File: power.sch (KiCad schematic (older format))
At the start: 60 parts, among them J5 VJ1, U1 LFE5U-85F-6BG381C, U3 TLV62569DBV, U4 TLV62569DBV, U5 TLV62569DBV

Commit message: Sync sch and pcb
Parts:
- removed D12: BAT54W, Diode_SMD:D_SOD-323_HandSoldering, symbol Device:D_Schottky
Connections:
- net labels removed: FTDI_nSUSPEND
- wire segments 395 -> 391
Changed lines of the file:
@@
 	7450 4700 6950 4700
 Wire Wire Line
-	3950 4950 4100 4950
-Wire Wire Line
 	4100 1050 4200 1050
 Wire Wire Line
@@
 Wire Wire Line
 	4850 4950 4850 4850
-Wire Wire Line
-	4100 4950 4100 5050
-Connection ~ 4100 4950
-Wire Wire Line
-	2850 4950 3650 4950
 Wire Wire Line
 	7750 1050 7750 1150
@@
 Wire Wire Line
 	2500 4950 2550 4950
-Text Label 2900 4950 0    60   ~ 0
-FTDI_nSUSPEND
 $Comp
 L Device:C C17
@@
 	1    0    0    -1
 $EndComp
-$Comp
-L Device:D_Schottky D12
-U 1 1 5AF673FF
-P 3800 4950
-F 0 "D12" H 3800 5050 50  0000 C CNN
-F 1 "BAT54W" H 3800 4850 50  0000 C CNN
-F 2 "Diode_SMD:D_SOD-323_HandSoldering" H 3800 4950 50  0001 C CNN
-F 3 "" H 3800 4950 50  0001 C CNN
-	1    3800 4950
-	-1   0    0    1
-$EndComp
 Text Notes 850  5050 0    60   ~ 0
 FTDI_nSLEEP is 2.5V\nD12 must be schottky
@@
 Wire Wire Line
 	2900 3700 2900 3800
-Wire Wire Line
-	4100 4950 4850 4950
 $EndSCHEMATC

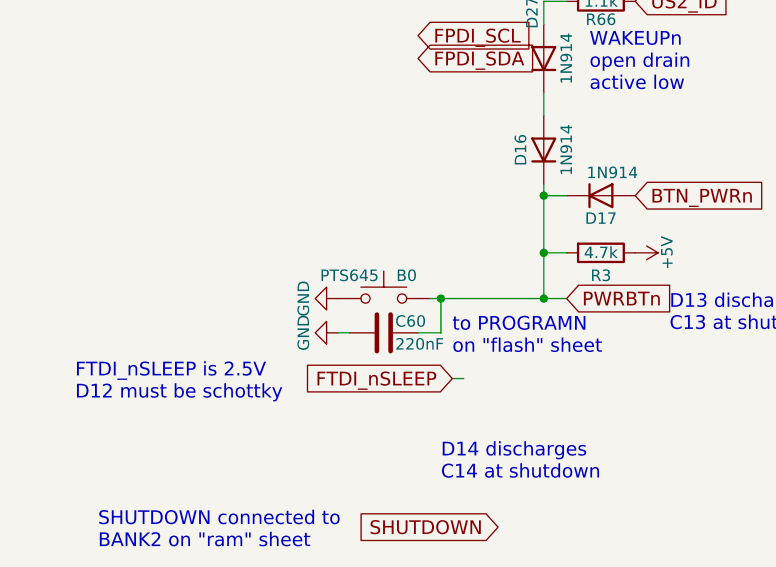
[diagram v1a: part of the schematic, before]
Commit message: Before removing USB port
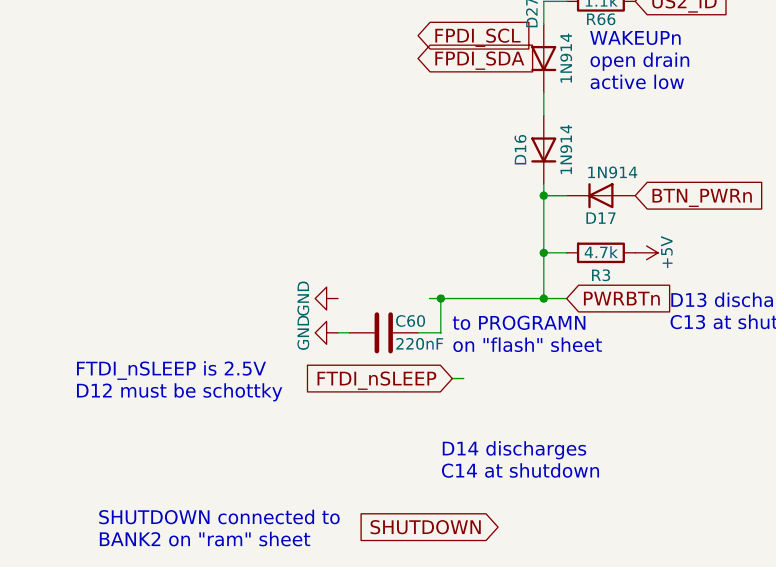
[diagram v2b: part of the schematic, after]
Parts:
- removed B0: PTS645, Button_Switch_SMD:SW_SPST_PTS645, symbol Switch:SW_Push
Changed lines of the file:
@@
 Text GLabel 3300 4150 2    60   Input ~ 0
 BTN_PWRn
-$Comp
-L Switch:SW_Push B0
-U 1 1 58E83FE0
-P 2200 4600
-F 0 "B0" H 2100 4700 50  0000 C CNN
-F 1 "PTS645" H 2350 4700 50  0000 C CNN
-F 2 "Button_Switch_SMD:SW_SPST_PTS645" H 2200 3400 50  0001 C CNN
-F 3 "http://www.ckswitches.com/media/1471/pts645.pdf" H 2200 3400 50  0001 C CNN
-F 4 "www.ckswitches.com" H 2200 4600 60  0001 C CNN "MNF1_URL"
-F 5 "PTS645SL50SMTR92 LFS" H 2200 4600 60  0001 C CNN "MPN"
-F 6 "611-PTS645SL50SMTR92" H 2200 4600 50  0001 C CNN "Mouser"
-F 7 "CKN9088CT-ND" H 2200 4600 50  0001 C CNN "Digikey"
-F 8 "15N4500" H 2200 4600 50  0001 C CNN "Newark"
-F 9 "79AH5908" H 2200 4600 50  0001 C CNN "Newar_k2"
-F 10 "C285463" H 2200 4600 50  0001 C CNN "LCSC"
-F 11 "0.09966$" H 2200 4600 50  0001 C CNN "price700_LCSC"
-F 12 "FSW001" H 2200 4600 50  0001 C CNN "Koncar"
-F 13 "T" H 2200 4600 50  0001 C CNN "Side"
-	1    2200 4600
-	-1   0    0    -1
-$EndComp
 Wire Wire Line
 	2350 2600 2450 2600
